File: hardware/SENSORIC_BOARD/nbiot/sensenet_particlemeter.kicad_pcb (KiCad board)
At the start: 2 copper layers, 63.6 x 72.3 mm, 102 parts, among them J1 CONN_01X01, J11 CONN_01X01, J13 BARREL_JACK, J17 CONN_01X01, J18 CONN_01X01, J19 CONN_01X01, J2 CONN_01X01, J20 CONN_01X01, J21 CONN_01X01, J3 CONN_01X01, J4 CONN_01X01, J5 CONN_01X01, J6 CONN_01X01, P1 SMA_mini, P2 SMA_mini, P3 CONN_02X12, Q1 Q_NMOS_GSD, SW1 SW_DPST, SW2 SW_DIP_x03, SW3 SW_DPST, U1 MC33063, U10 bme280_barebone, U2 stm32f072, U3 QUECTEL_BC95, U4 SIM, U5 CAT24C02, U6 MC33063, U7 M10578-A2, U8 usb_femalee, Y1 8MHz

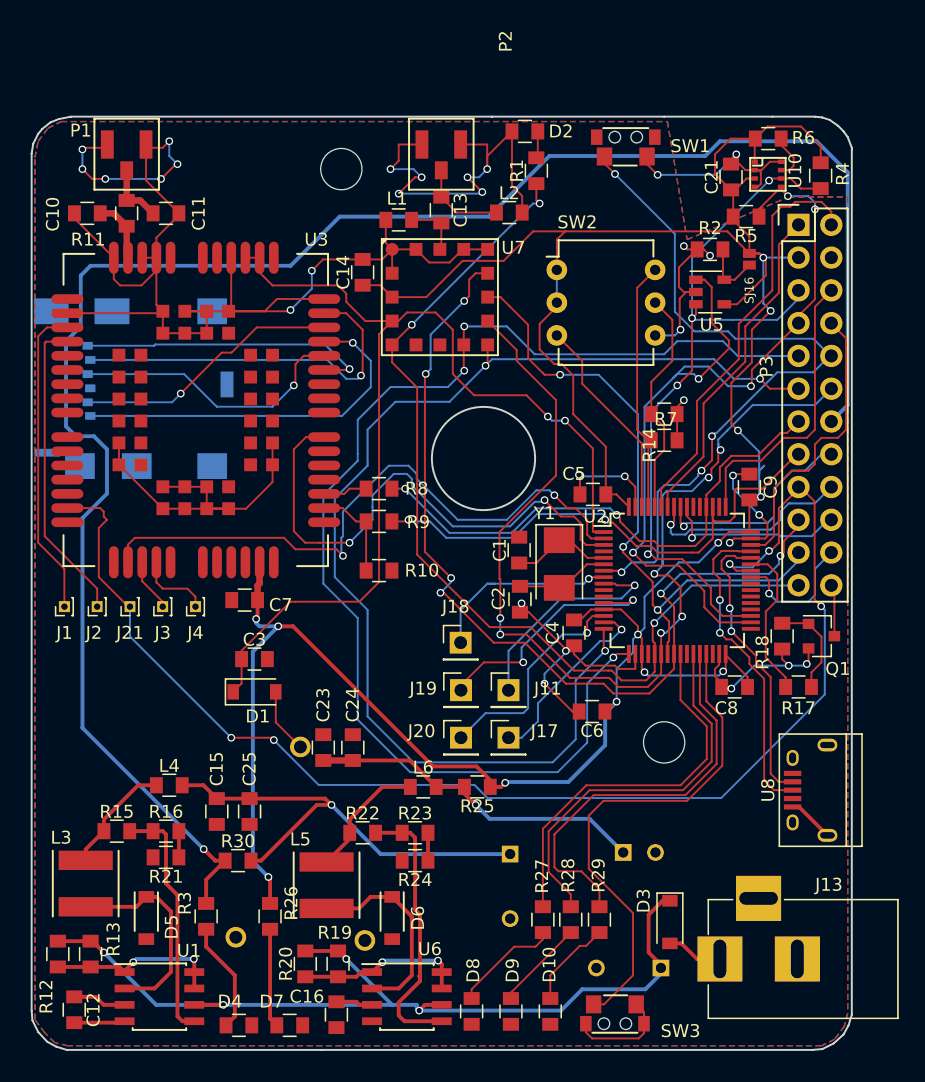
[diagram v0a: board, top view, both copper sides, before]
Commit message: pred displayem
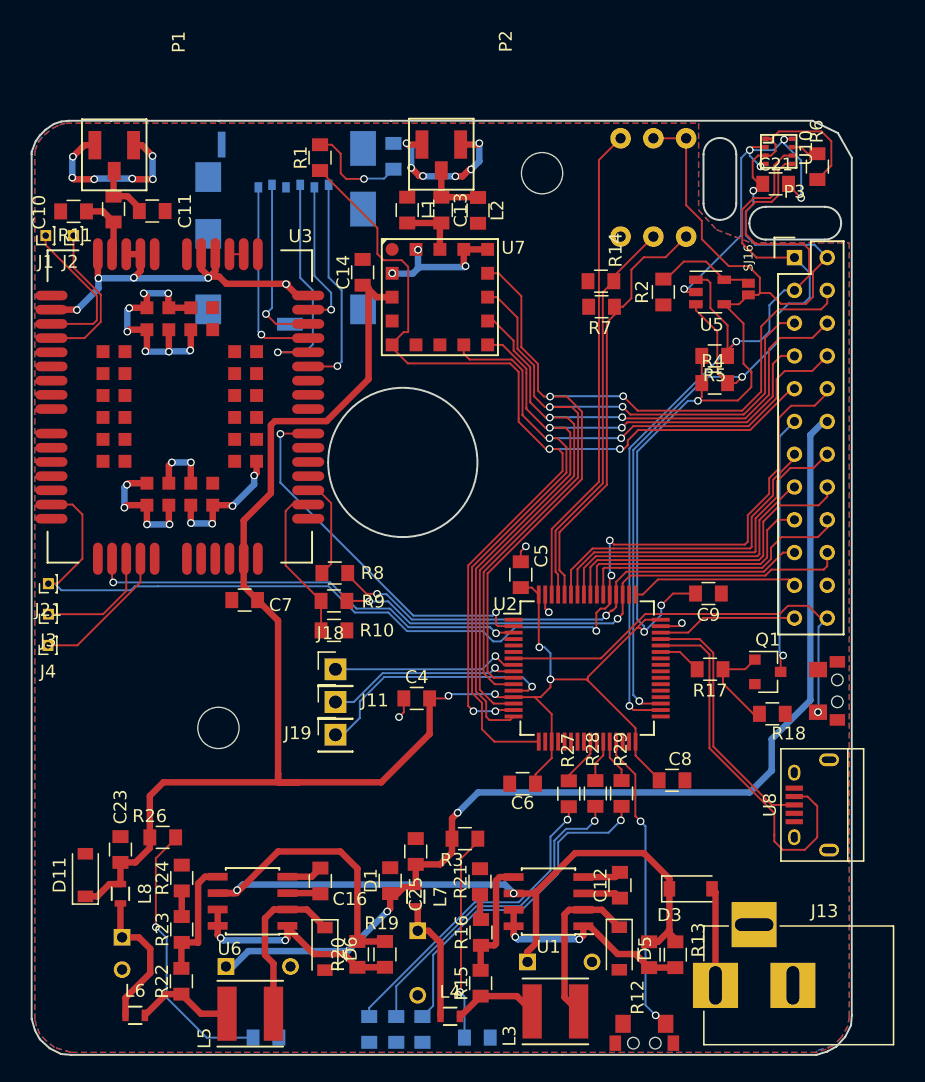
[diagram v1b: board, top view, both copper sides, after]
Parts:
- removed ?: , koksovna:drawing
- removed BT1: Battery_Cell, SNPM:BAT-CR2032_bottom
- removed C1, C2: 4.3p, SNPM:SMD_0805
- removed C24: 220n, SNPM:SMD_0805
- removed C3: C, SNPM:SMD_0805
- removed J17, J20: CONN_01X01, SNPM:Pin_Header_Straight_1x01_Pitch2.54mm
- removed R25, R30: 0R1, SNPM:SMD_0805
- removed Y1: 8MHz, Crystals:Crystal_SMD_5032-2pin_5.0x3.2mm
- added D11: SM2T3V3A, SNPM:D_SOD-123, F.Cu at (136.2, 112.2)
- added L7: FBMH1608HL601-T, Resistors_SMD:R_0603, F.Cu at (161.8, 113.9)
- added L8: FBMH1608HL601-T, Resistors_SMD:R_0603, F.Cu at (139.0, 113.7)
- C15: value 1u -> 1000u; footprint SNPM:SMD_0805 -> SNPM:C_Radial_D10_L16_P5_bottom
- D1: value D_Schottky -> PTVS3V3S1UR,115; footprint SNPM:D_SOD-123 -> SNPM:SMD_0805
- D10, D2, D8, D9: footprint SNPM:SMD_0805 -> SNPM:SMD_0805_bottom
- D4: value LED -> red LED; footprint SNPM:SMD_0805 -> SNPM:SMD_0805_bottom
- D5, D6: footprint Diodes_SMD:SOD-123 -> SNPM:D_SOD-123
- D7: value LED -> green LED; footprint SNPM:SMD_0805 -> SNPM:SMD_0805_bottom
- L3, L5: footprint Inductors:Inductor_Taiyo-Yuden_NR-50xx -> SNPM:Inductor_Taiyo-Yuden_NR-50xx
- L4, L6: value 1uH -> FBMH1608HL601-T; footprint SNPM:SMD_0805 -> Resistors_SMD:R_0603
- P3: footprint Pin_Headers:Pin_Header_Straight_2x12 -> SNPM:Pin_Header_Straight_2x12
- Q1: footprint TO_SOT_Packages_SMD:SOT-23 -> SNPM:SOT-23
- R16: value 9.1k -> 10k
- R22: value 18k -> 8k2
- R23: value 11k -> 5k6
- R26: value 5k6 -> 1k
- R3: value 5k6 -> 8k2
- SW1, SW3: footprint SNPM:edge_switch -> SNPM:edge_switch_bot
- SW2: footprint Housings_DIP:DIP-6_W7.62mm -> SNPM:DIP-6_W7.62mm_bot
- U1: footprint Housings_SOIC:SOIC-8_3.9x4.9mm_Pitch1.27mm -> SNPM:SOIC-8_3.9x4.9mm_Pitch1.27mm
- moved SW1 46.3 mm to (193.5, 98.0), turned to 270 degrees
- moved R12 45.8 mm to (179.9, 118.4)
- moved R13 45.3 mm to (182.0, 118.4)
- moved C12 43.4 mm to (177.7, 113.0), turned to 90 degrees
- moved C18 39.4 mm to (139.1, 117.1), turned to 270 degrees
- moved L3 37.7 mm to (172.7, 122.8), turned to 180 degrees
- moved D5 36.7 mm to (177.6, 117.9)
- moved J5 34.6 mm to (146.6, 100.8)
- moved U1 31.0 mm to (172.1, 114.3), turned to 180 degrees
- moved R15 30.6 mm to (166.9, 120.6), turned to 90 degrees
- moved J2 28.8 mm to (135.3, 62.7)
- moved J1 28.8 mm to (133.2, 62.7)
- moved L6 28.5 mm to (140.1, 123.1)
- moved L4 28.2 mm to (164.5, 123.2)
- moved R16 25.6 mm to (166.9, 116.7), turned to 90 degrees
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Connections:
- C15 pad 1: Net-(C15-Pad1) -> +5V
- C17 pad 1: Net-(C15-Pad1) -> Net-(C17-Pad1)
- C23 pad 1: Net-(C18-Pad1) -> +3V3
- C25 pad 1: Net-(C15-Pad1) -> +5V
- D1 pad 1: batt -> +5V
- D1 pad 2: Net-(BT1-Pad1) -> GND
- L4 pad 1: Net-(L3-Pad2) -> Net-(C17-Pad1)
- L4 pad 2: Net-(C15-Pad1) -> Net-(L3-Pad2)
- L6 pad 1: Net-(L5-Pad2) -> Net-(C18-Pad1)
- L6 pad 2: Net-(C18-Pad1) -> Net-(L5-Pad2)
- P3 pad 1: USART_debug_tx -> i2c_sda
- P3 pad 10: reset -> WIRELESS_reset
- P3 pad 11: UART_GPS_TX -> NMOS
- P3 pad 12: gps_standby -> +5V
- P3 pad 13: Rx -> USART_debug_rx
- P3 pad 14: +5V -> USART_debug_tx
- P3 pad 15: Tx -> PM_SDI
- P3 pad 17: WIRELESS_reset -> PM_SCK
- P3 pad 18: PM_SDI -> PM_SS
- P3 pad 19: gps_pulses -> Rx
- P3 pad 2: USART_debug_rx -> +3V3
- P3 pad 20: PM_SCK -> Tx
- P3 pad 21: gps_reset -> SWD_CLK
- P3 pad 22: PM_SS -> GND
- P3 pad 23: gps_fix -> SWD_DIO
- P3 pad 24: Net-(P3-Pad24) -> reset
- P3 pad 3: +3V3 -> i2c_scl
- P3 pad 4: GND -> gps_pulses
- P3 pad 5: i2c_sda -> gps_reset
- P3 pad 6: SWD_CLK -> gps_standby
- P3 pad 7: i2c_scl -> UART_GPS_TX
- P3 pad 8: SWD_DIO -> UART_GPS_RX
- P3 pad 9: UART_GPS_RX -> gps_fix
- Q1 pad 3: Net-(P3-Pad24) -> NMOS
- R14 pad 2: BOOT_0 -> BOOT_signal
- R7 pad 2: BOOT_signal -> BOOT_0
- SW2 pad 1: +3V3 -> BOOT_0
- SW2 pad 2: +3V3 -> BOOT_signal
- SW2 pad 3: debug_on_off -> GND
- SW2 pad 4: GND -> debug_on_off
- SW2 pad 5: BOOT_0 -> +3V3
- SW2 pad 6: BOOT_signal -> +3V3
- U2 pad 1: batt -> (no net)
- U2 pad 10: (no net) -> gps_pulses
- U2 pad 11: (no net) -> gps_reset
- U2 pad 14: Net-(J20-Pad1) -> gps_standby
- U2 pad 15: Net-(J17-Pad1) -> gps_fix
- U2 pad 2: NETLIGHT -> RI
- U2 pad 21: gps_fix -> (no net)
- U2 pad 22: gps_standby -> (no net)
- U2 pad 23: gps_reset -> (no net)
- U2 pad 24: gps_pulses -> (no net)
- U2 pad 3: RI -> NETLIGHT
- U2 pad 41: PM_SS -> (no net)
- U2 pad 42: WIRELESS_reset -> (no net)
- U2 pad 5: Net-(C1-Pad1) -> (no net)
- U2 pad 53: (no net) -> WIRELESS_reset
- U2 pad 54: (no net) -> PM_SS
- U2 pad 6: Net-(C2-Pad1) -> (no net)
- U7 pad 14: batt -> (no net)
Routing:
- net GND: track 262.3 -> 153.9 mm, vias 31 -> 46
- net batt: track 81.1 -> 1.10 mm, vias 2 -> 0
- net +5V: track 142.3 -> 80.9 mm, vias 1 -> 2
- net Net-(C15-Pad1): track 35.7 -> 0.00 mm, vias 1 -> 0
- net UART_GPS_TX: track 90.6 -> 61.5 mm, vias 3 -> 2
- net Net-(R29-Pad1): track 32.0 -> 3.40 mm
- net UART_GPS_RX: track 97.0 -> 68.7 mm, vias 3 -> 2
- net Net-(R28-Pad1): track 30.4 -> 3.27 mm
- net Net-(R27-Pad1): track 30.0 -> 3.73 mm
- net +3V3: track 230.9 -> 254.9 mm, vias 13 -> 8
- net reset: track 56.7 -> 34.4 mm, vias 4 -> 1
- net debug_on_off: track 16.0 -> 37.6 mm
- net NMOS: track 0.00 -> 20.1 mm, vias 0 -> 1
- net Net-(D10-Pad2): track 7.04 -> 26.5 mm, vias 0 -> 1
- net Net-(D9-Pad2): track 7.03 -> 25.6 mm, vias 0 -> 1
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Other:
- board size 63.6 x 72.3 mm -> 63.6 x 72.4 mm
- net class Default: trace_width 0.15 -> 0.5
- rule pad_to_mask_clearance: 0.2 -> 0.15
